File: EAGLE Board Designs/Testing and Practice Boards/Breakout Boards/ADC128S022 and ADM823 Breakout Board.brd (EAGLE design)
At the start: 160 x 100 mm, 5 parts

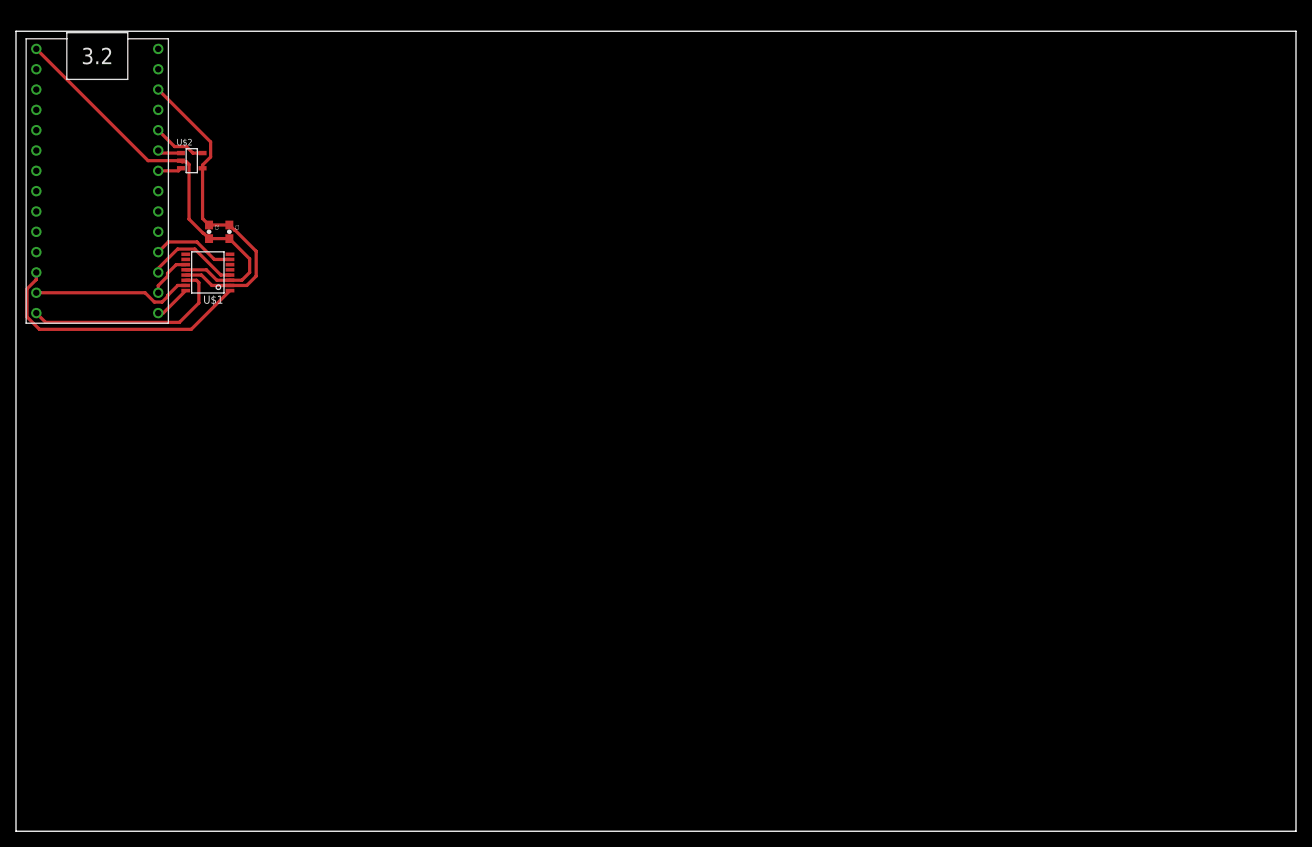
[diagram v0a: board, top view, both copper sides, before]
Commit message: update schematic and board based on feedback
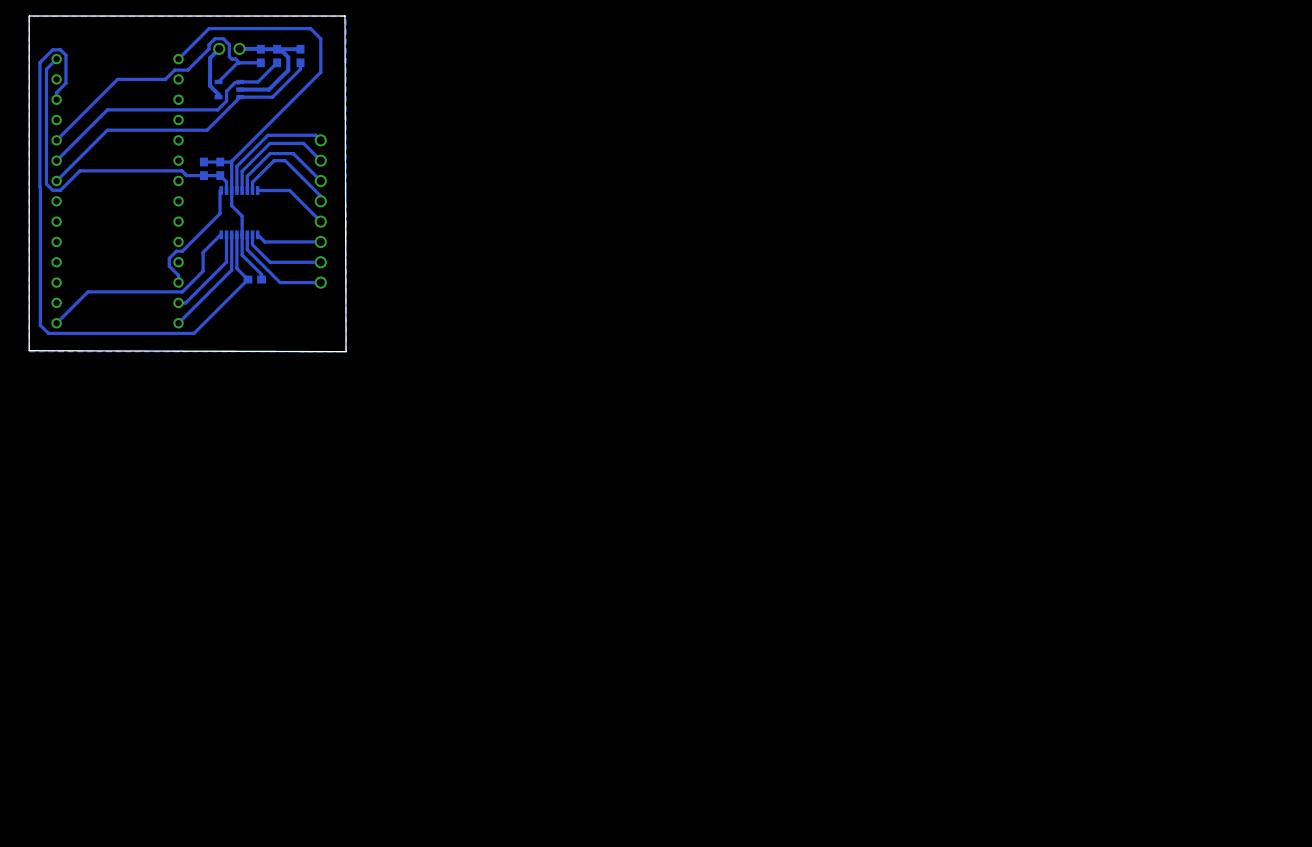
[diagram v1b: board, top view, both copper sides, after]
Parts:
- added C3: 0.1uF, HyTechDevices:0603-CAP
- added JP1, JP2: (no value), HyTechDevices:1X04
- added JP3: M02, HyTechDevices:1X02
- added R1: 1M, HyTechDevices:0603-RES
- added R2, R3: 10k, HyTechDevices:0603-RES
- moved U$3 20.4 mm to (21.6, 62.2), flipped to the bottom
- moved U$2 10.1 mm to (26.7, 92.7), flipped to the bottom
- moved U$1 8.52 mm to (27.9, 77.5), flipped to the bottom, turned to 180 degrees
- moved C1 7.96 mm to (25.5, 82.8), flipped to the bottom
- moved C2 7.90 mm to (23.5, 82.8), flipped to the bottom
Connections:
- new net +5V: C1.2, C2.2, U$1.2, U$3.VIN
- new net N$1: JP1.1, U$1.4
- new net N$2: JP1.2, U$1.5
- new net N$3: JP1.3, U$1.6
- new net N$4: JP1.4, U$1.7
- new net N$5: JP2.1, U$1.8
- new net N$6: JP2.2, U$1.9
- new net N$7: JP2.3, U$1.10
- new net N$8: JP2.4, U$1.11
- new net WATCHDOG_3V3: JP3.2, U$2.4
- new net WATCHDOG_GND: JP3.1, R1.1, R2.1, R3.2, U$2.2
- net !MR!: now also R1.2
- net !RESET!: now also R3.1
- net +3V3: now also C3.1; no longer C1.1, C2.1, U$1.2, U$2.4
- net GND: now also C1.1, C2.1, C3.2; no longer C1.2, C2.2, U$2.2
- net IN0: no longer U$1.4
- net IN3: no longer U$1.7
- net IN7: no longer U$1.11
- net WDI: now also R2.2
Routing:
- net +5V: track 0.00 -> 41.6 mm
- net +3V3: track 40.6 -> 78.4 mm
- net !MR!: track 2.97 -> 37.1 mm
- net !RESET!: track 2.97 -> 33.3 mm
- net WDI: track 6.73 -> 36.8 mm
- net SCLK: track 4.59 -> 26.5 mm
- net CS: track 34.1 -> 15.1 mm
- net WATCHDOG_GND: track 0.00 -> 17.7 mm
- net N$1: track 0.00 -> 15.4 mm
- net N$2: track 0.00 -> 14.6 mm
- net N$3: track 0.00 -> 13.6 mm
- net N$4: track 0.00 -> 13.2 mm
- net N$8: track 0.00 -> 12.8 mm
- net SDI: track 26.1 -> 13.8 mm
- net IN0: track 11.8 -> 0.00 mm
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- added copper zone on layer 16, net GND
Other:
- board size 160 x 100 mm -> 39.6 x 42 mm

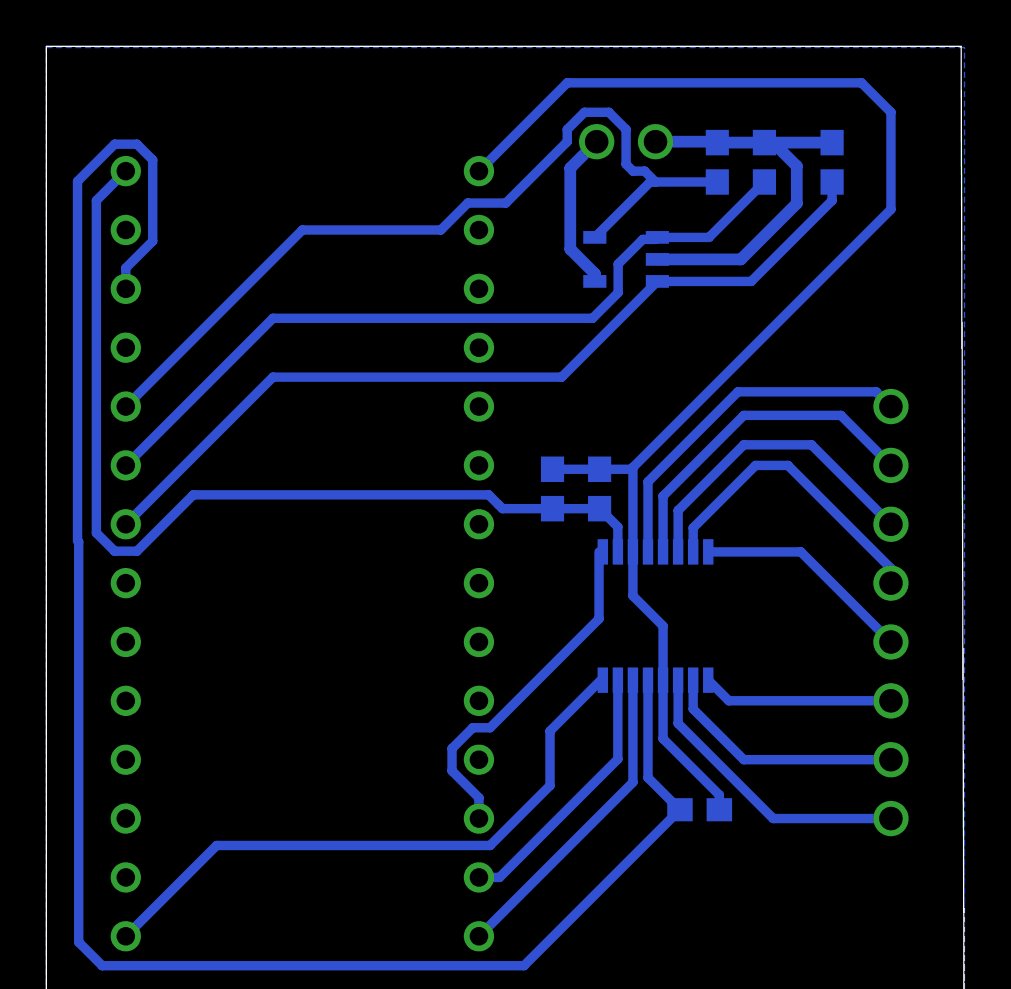
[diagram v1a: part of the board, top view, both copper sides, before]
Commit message: ready for manufacturing
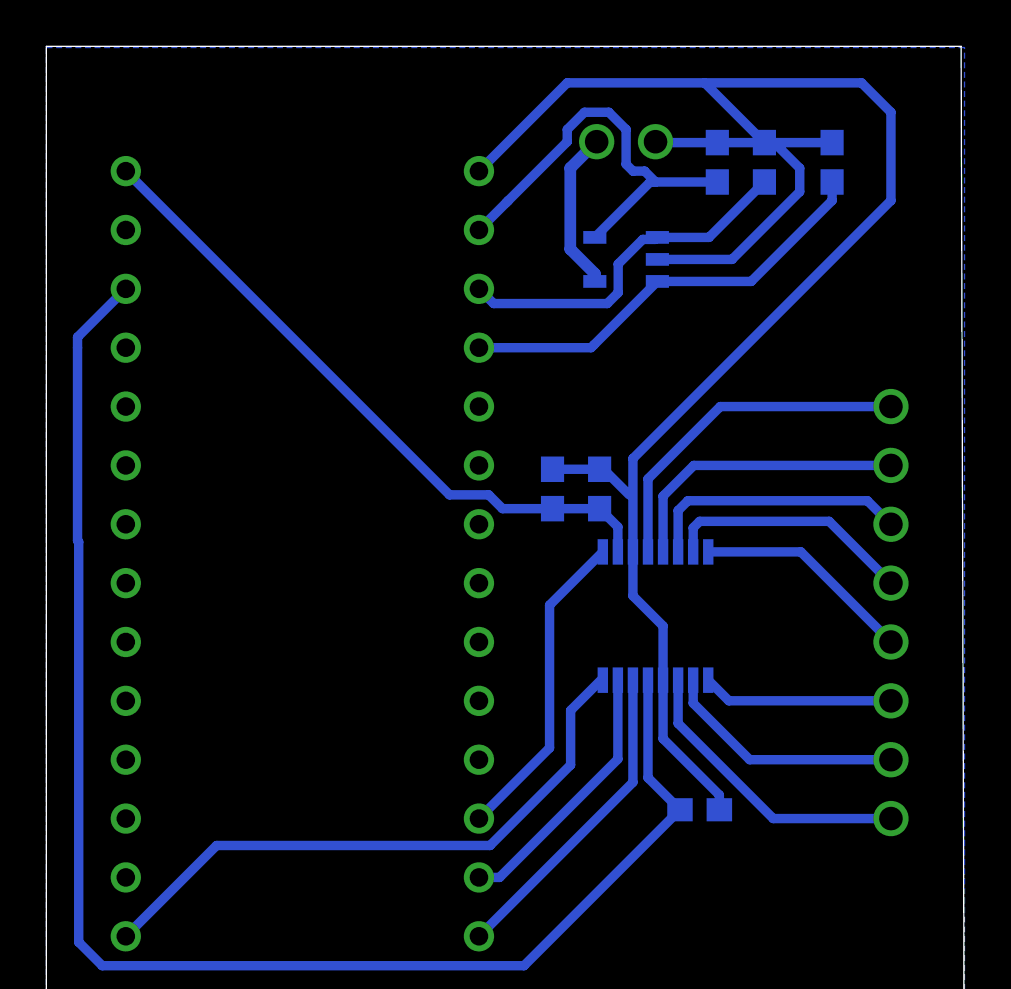
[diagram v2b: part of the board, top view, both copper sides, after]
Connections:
- removed net IN0: U$3.A1
- removed net IN3: U$3.A2
- removed net IN7: U$3.A0
- removed net WATCHDOG_GND: JP3.1, R1.1, R2.1, R3.2, U$2.2
- net !MR!: now also U$3.D2; no longer U$3.A6
- net !RESET!: now also U$3.D1(TX1); no longer U$3.A7
- net GND: now also JP3.1, R1.1, R2.1, R3.2, U$2.2
- net WDI: now also U$3.D0(RX1); no longer U$3.A8
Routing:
- net GND: track 59.6 -> 81.8 mm
- net !MR!: track 37.1 -> 18.7 mm
- net WDI: track 36.8 -> 18.6 mm
- net !RESET!: track 33.3 -> 15.5 mm
- net WATCHDOG_GND: track 17.7 -> 0.00 mm
- net +3V3: track 78.4 -> 64.4 mm
- net +5V: track 41.6 -> 28.7 mm
- net N$4: track 13.2 -> 10.8 mm
- net N$3: track 13.6 -> 11.6 mm
- net N$2: track 14.6 -> 12.8 mm
- net CS: track 15.1 -> 13.7 mm
